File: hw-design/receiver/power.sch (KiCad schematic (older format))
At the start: 14 parts, among them P1 CONN_01X03, SW2 power, U5 MCP73833, U6 AP1117D33

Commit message: Skończona rewizja r1, wysłane do satlanfd
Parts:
- SW2: footprint w_switch:PCB_PUSH -> w_pin_strip:pin_socket_2; Opis (none) -> Włącznik zasilania, kołyskowy.
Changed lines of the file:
@@
 F 0 "SW2" H 6700 3225 50  0000 C CNN
 F 1 "power" H 6700 3300 50  0000 C CNN
-F 2 "w_switch:PCB_PUSH" H 6700 3125 60  0001 C CNN
-F 3 "" H 6700 3125 60  0000 C CNN
+F 2 "w_pin_strip:pin_socket_2" H 6700 3125 60  0001 C CNN
+F 3 "http://lispol.pl/product,2183,wylacznik_kolyskowy_mini_czarny.html" H 6700 3125 60  0001 C CNN
+F 4 "Włącznik zasilania, kołyskowy." H 6700 3125 60  0001 C CNN "Opis"
 	1    6700 3125
 	1    0    0    -1

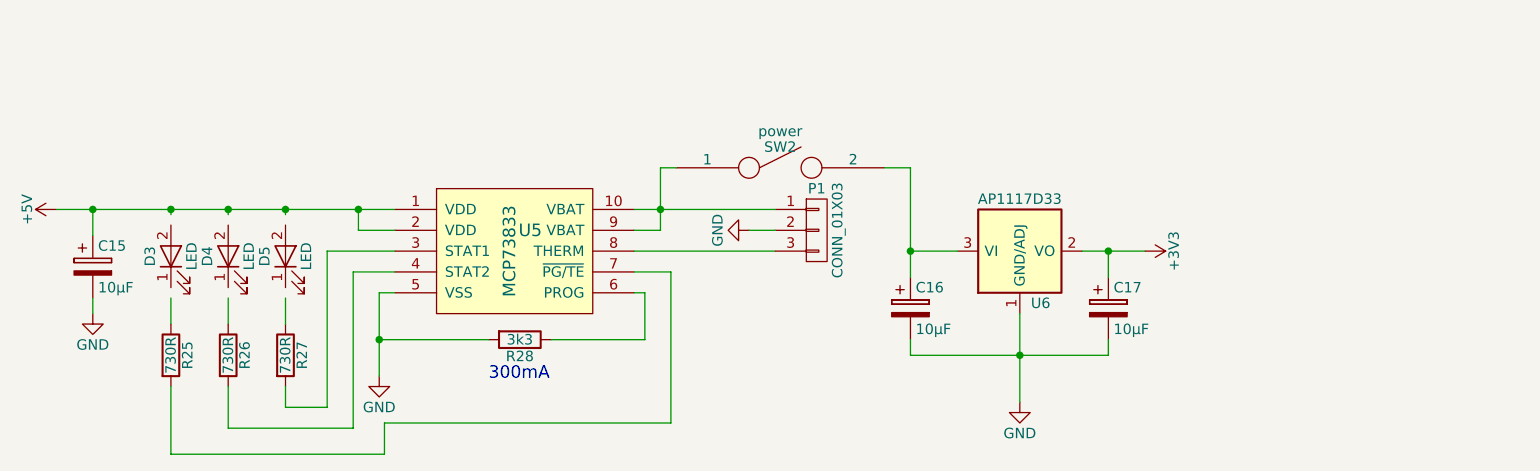
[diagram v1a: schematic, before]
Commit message: Revision 2
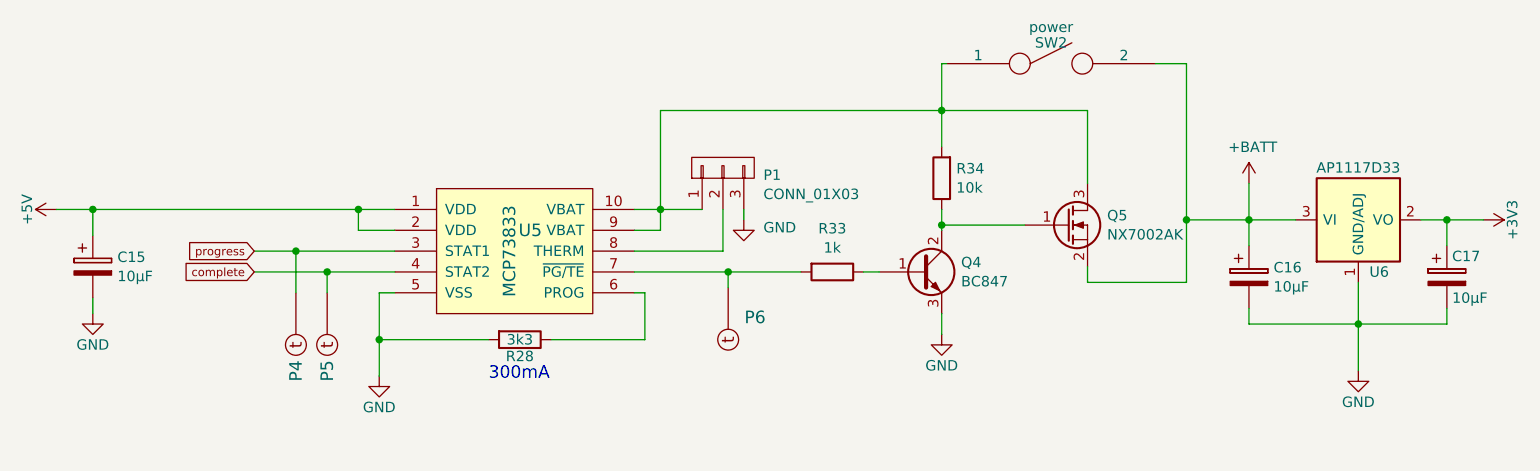
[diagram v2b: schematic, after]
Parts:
- removed D3: LED, w_indicators:led_3mm_yellow, symbol LED
- removed D4: LED, w_indicators:led_3mm_green, symbol LED
- removed D5: LED, w_indicators:led_3mm_red, symbol LED
- removed R25, R26, R27: 730R, w_smd_resistors:r_0603, symbol R
- added P4, P5, P6: test-double, iwasz:testpad-2p, symbol test-double
- added Q4: BC847, w_smd_trans:sot23, symbol Q_NPN_BCE
- added Q5: NX7002AK, iwasz:sot23-pins123-ccw, symbol Q_NMOS_GSD
- added R33: 1k, w_smd_resistors:r_0603, symbol R
- added R34: 10k, w_smd_resistors:r_0603, symbol R
- C15, C16, C17: footprint w_smd_cap:c_tant_A -> w_smd_cap:c_tant_B
- P1: footprint w_conn_df13:df13-3p-125dsa -> w_pin_strip:pin_strip_3
- SW2: footprint w_pin_strip:pin_socket_2 -> w_pin_strip:pin_strip_2
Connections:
- net labels added: +BATT, complete, progress
- wire segments 46 -> 43
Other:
- moved on the sheet: C16, C17, P1, SW2, U6
